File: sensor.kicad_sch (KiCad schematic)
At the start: 1 part, among them IC1 USR-ES1

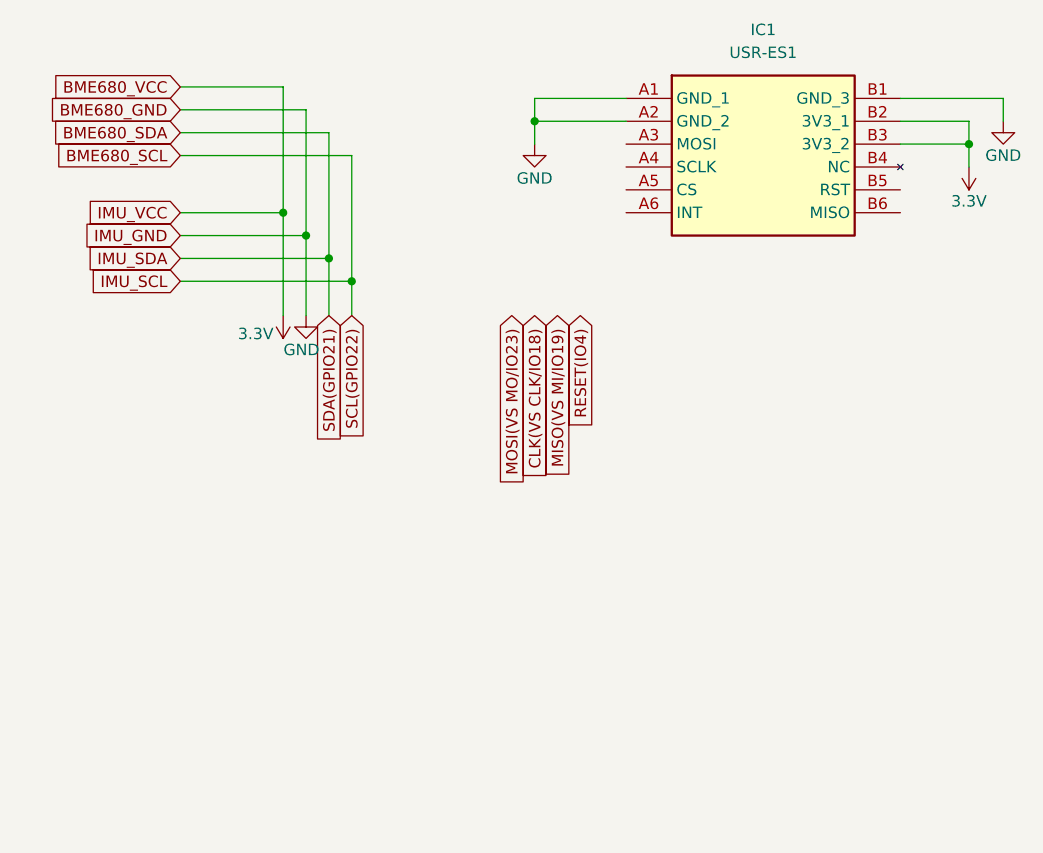
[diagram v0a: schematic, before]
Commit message: breadboard test
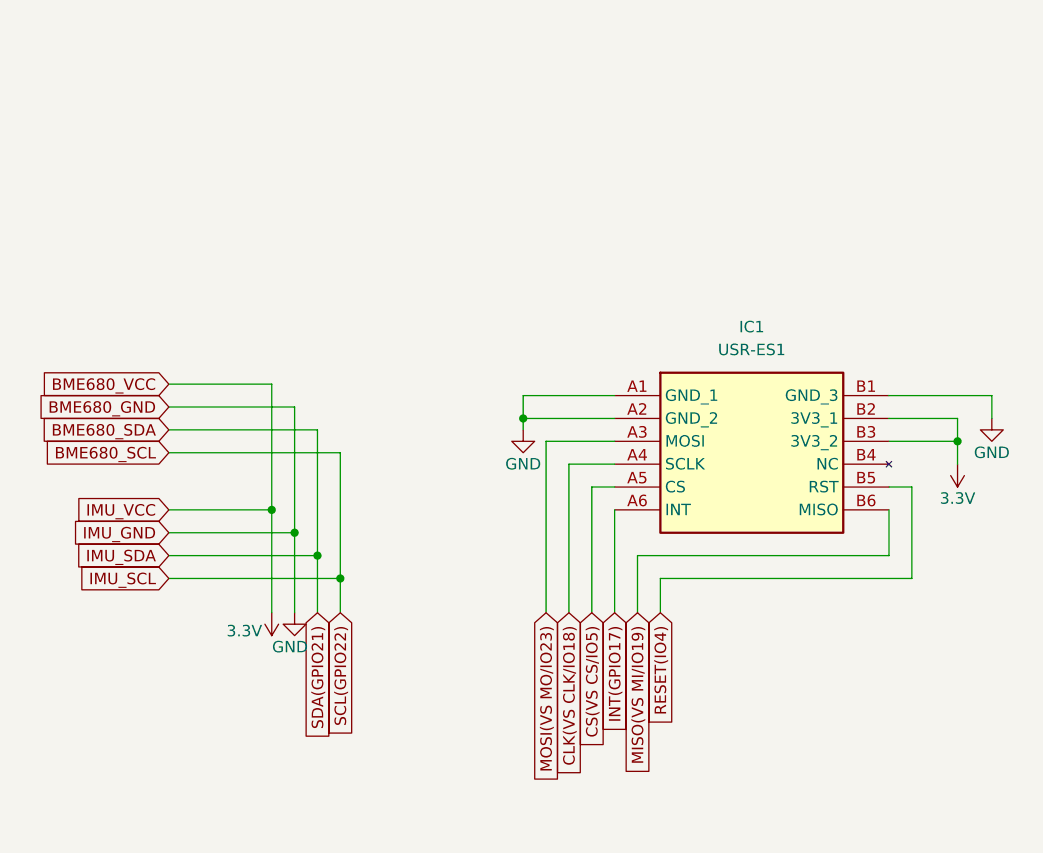
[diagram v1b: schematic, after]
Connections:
- net CLK(VS CLK/IO18): now also IC1.A4 (SCLK)
- net MISO(VS MI/IO19): now also IC1.B6 (MISO)
- net MOSI(VS MO/IO23): now also IC1.A3 (MOSI)
- net RESET(IO4): now also IC1.B5 (RST)
- net CS(VS CS/IO5): now reaches IC1.A5 (CS)
- net INT(GPIO17): now reaches IC1.A6 (INT)
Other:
- moved on the sheet: IC1
